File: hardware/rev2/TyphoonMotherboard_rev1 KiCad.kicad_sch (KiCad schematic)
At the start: 80 parts, among them J1 Conn_02x04_Odd_Even, J2 Conn_01x04_Pin, J3 UJ20-C-H-C-4-SMT-TR, J5 Conn_01x02_Pin, J6 Conn_01x02_Pin, J7 Conn_01x04_Pin, SW1 SW_Push, SW2 SW_Push, SW3 SW_Push, U1 USBLC6-2SC6, U2 ESP32-S3-WROOM-1, U3 SN65HVD233, U4 BQ25798RQMR, U5 TPS62130, U6 TPS62130

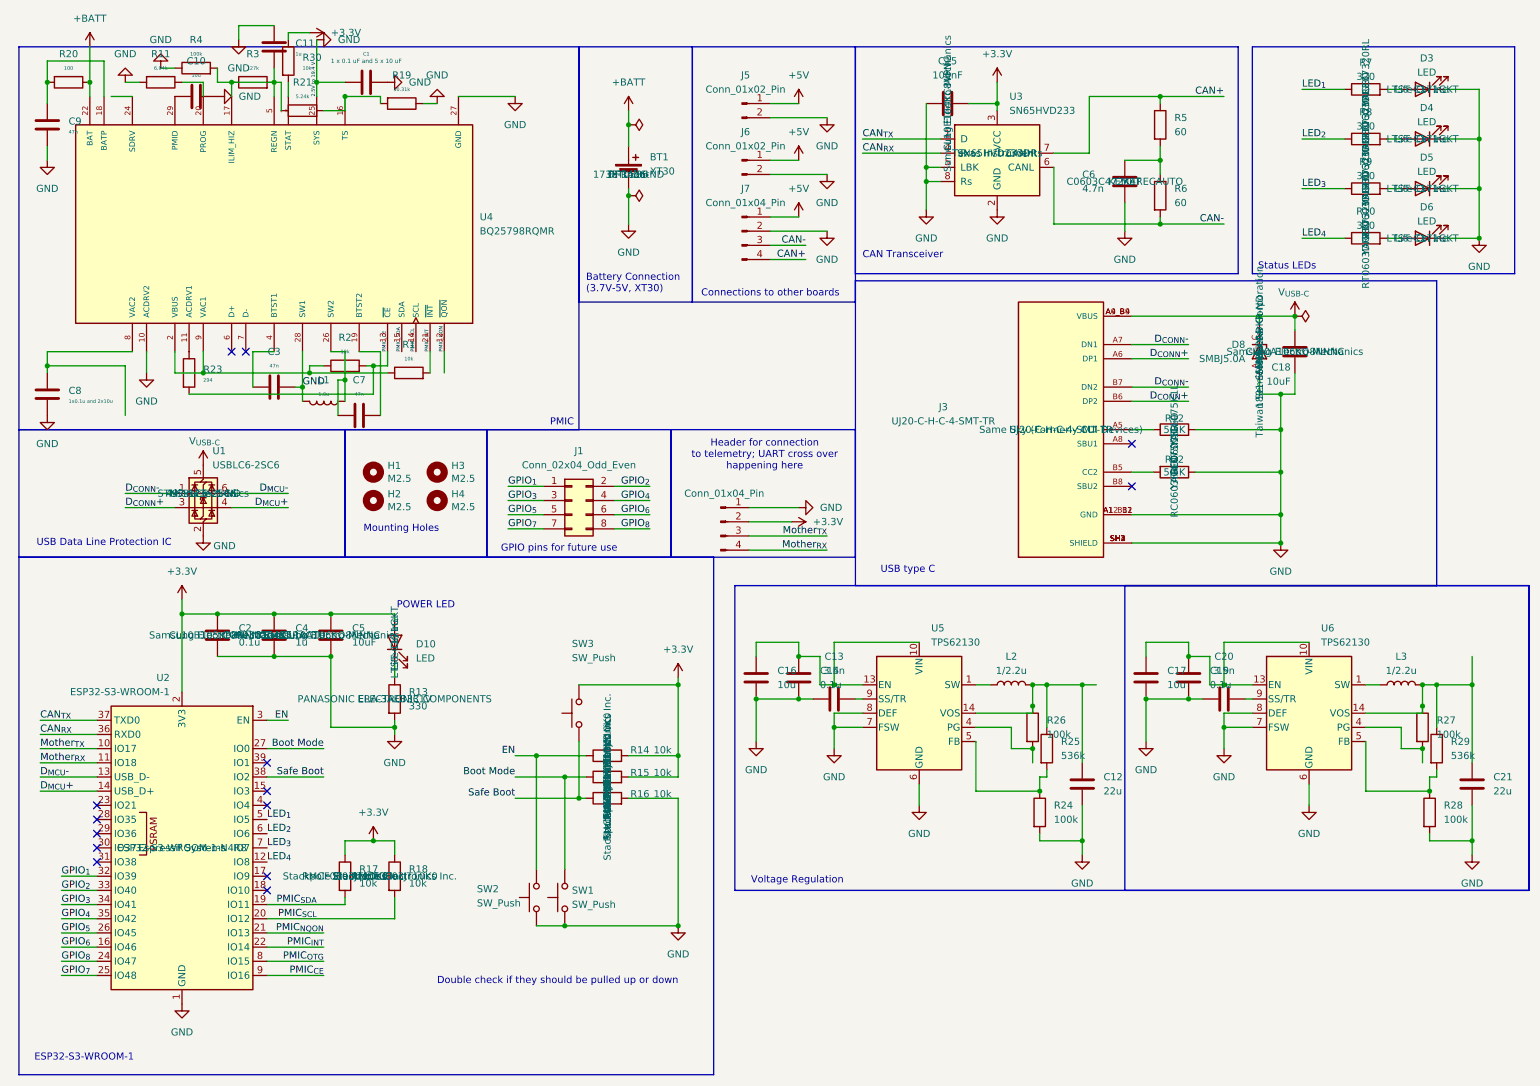
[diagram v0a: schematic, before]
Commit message: Reviewed the Schematic making PCB
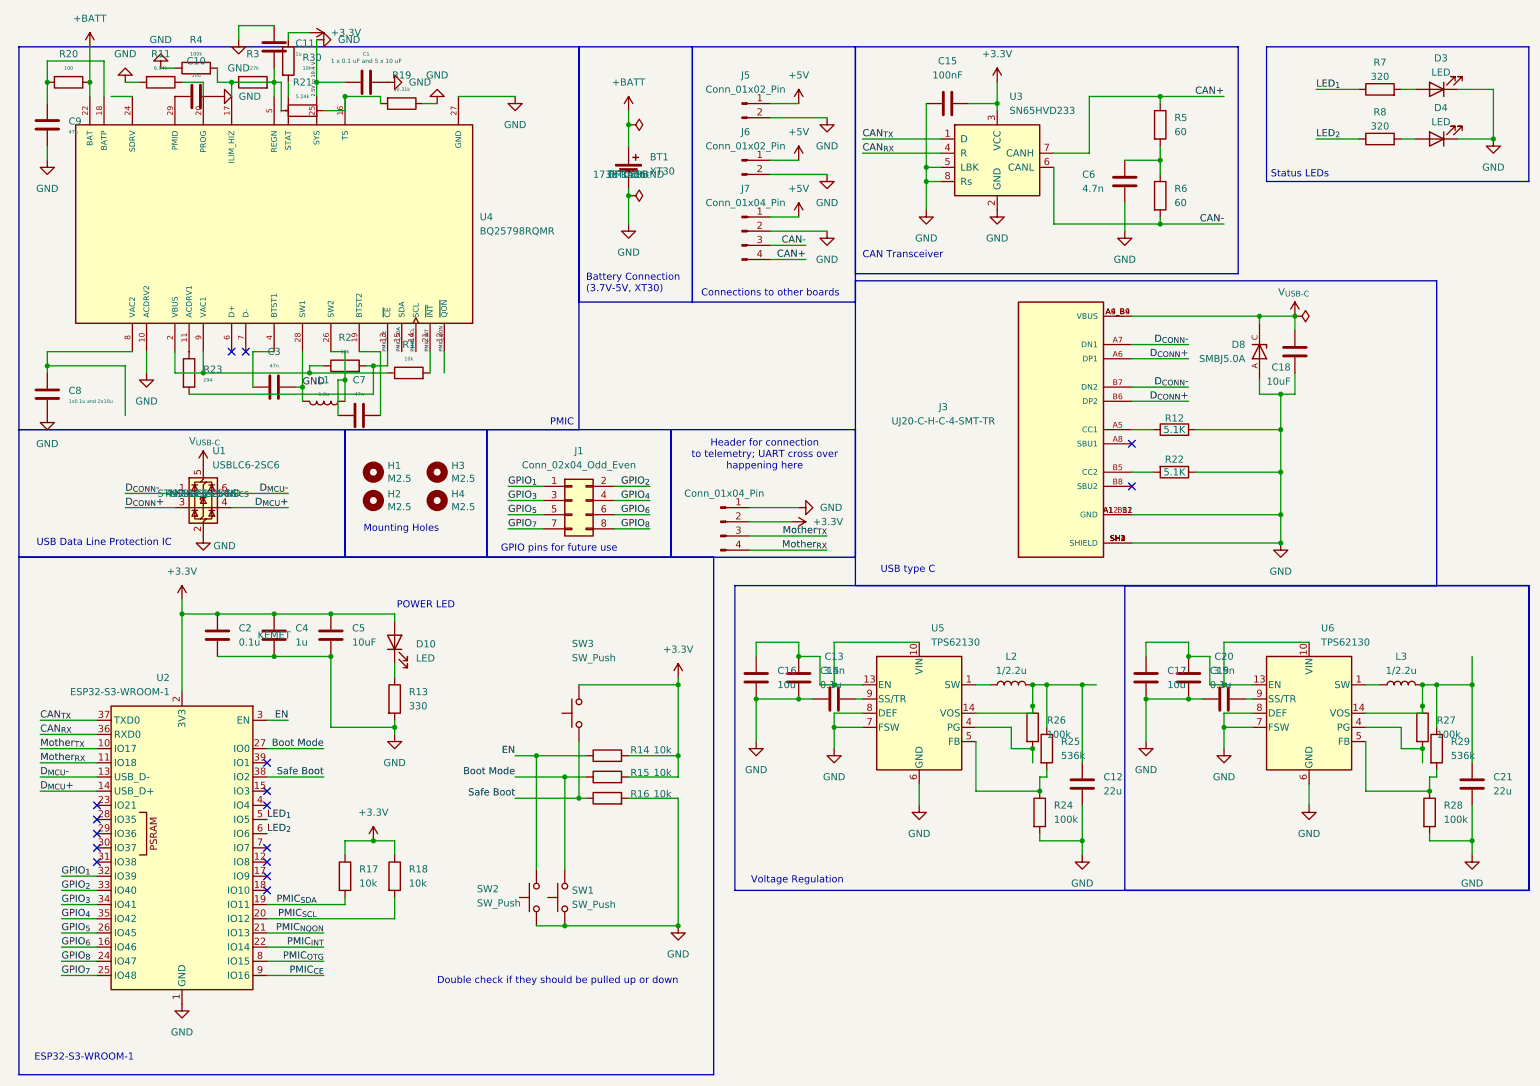
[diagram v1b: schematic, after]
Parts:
- removed D5, D6: LED, LED_SMD:LED_0805_2012Metric, symbol Device:LED
- removed R10, R9: 320, Resistor_SMD:R_0603_1608Metric, symbol Device:R
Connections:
- net LED_{3}: no longer names the net of U2.7 (IO7)
- net LED_{4}: no longer names the net of U2.12 (IO8)
- no-connect marks 14 -> 16
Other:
- moved on the sheet: D3, D4, R7, R8
